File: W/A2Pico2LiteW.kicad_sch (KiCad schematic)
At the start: 11 parts, among them U1 RPI-Pico2W, U2 74LVC1G11

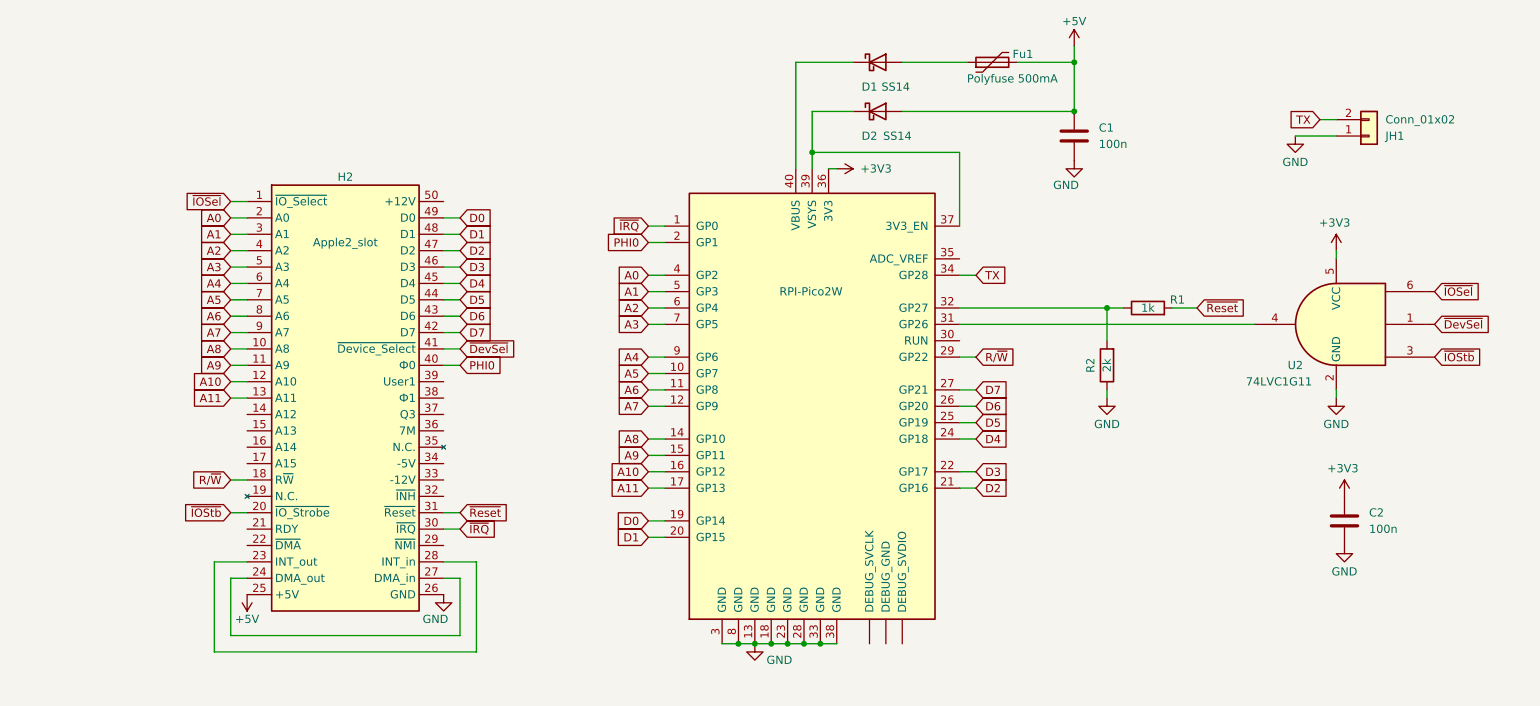
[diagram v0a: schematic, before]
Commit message: Add files via upload
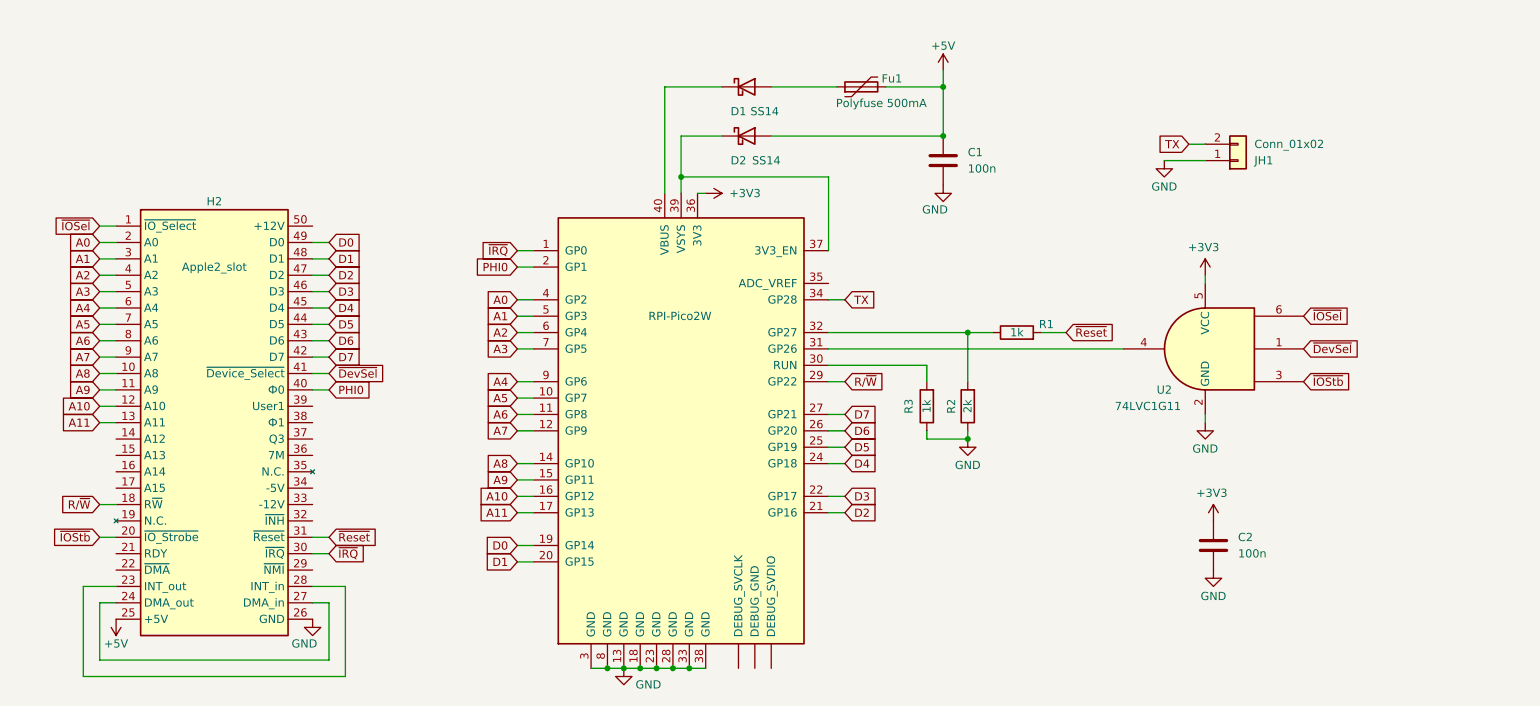
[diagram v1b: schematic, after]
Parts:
- added R3: 1k, Resistor_SMD:R_0402_1005Metric_Pad0.72x0.64mm_HandSolder, symbol Device:R
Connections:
- net GND: now also R3.1
- net at U1.30 (RUN): now also R3.2
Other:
- moved on the sheet: C1, C2, D1, D2, Fu1, H2, JH1, R1, R2, U2
